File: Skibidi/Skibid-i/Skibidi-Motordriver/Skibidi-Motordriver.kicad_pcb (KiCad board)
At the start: 2 copper layers, 65.5 x 94 mm, 13 parts, among them J1 XT90, J2 XT90, J5 XT90, J7 Screw_Terminal_01x02, J8 Screw_Terminal_01x02, Q1 IGBT, Q2 IGBT, Q3 IGBT, Q4 IGBT, Q5 IGBT, Q6 IGBT, Q7 IGBT, Q8 IGBT

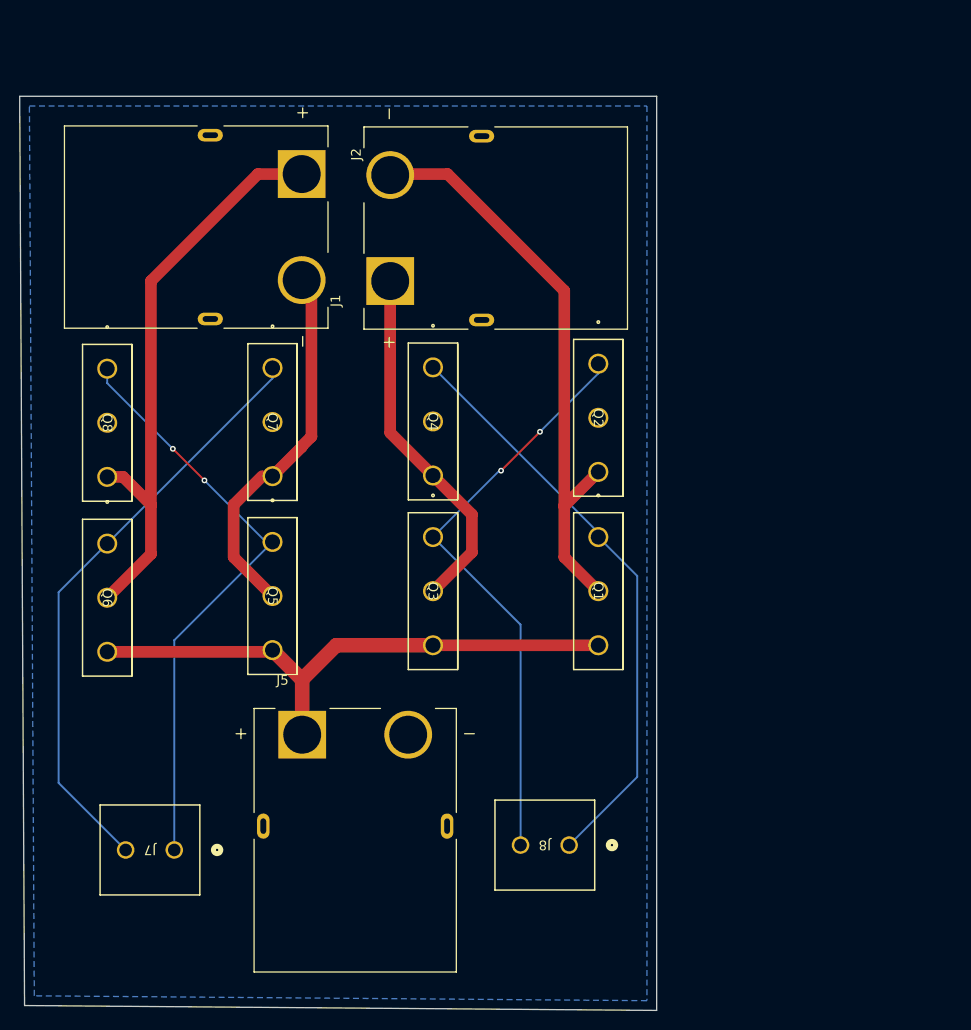
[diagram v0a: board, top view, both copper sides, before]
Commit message: finish motor driver
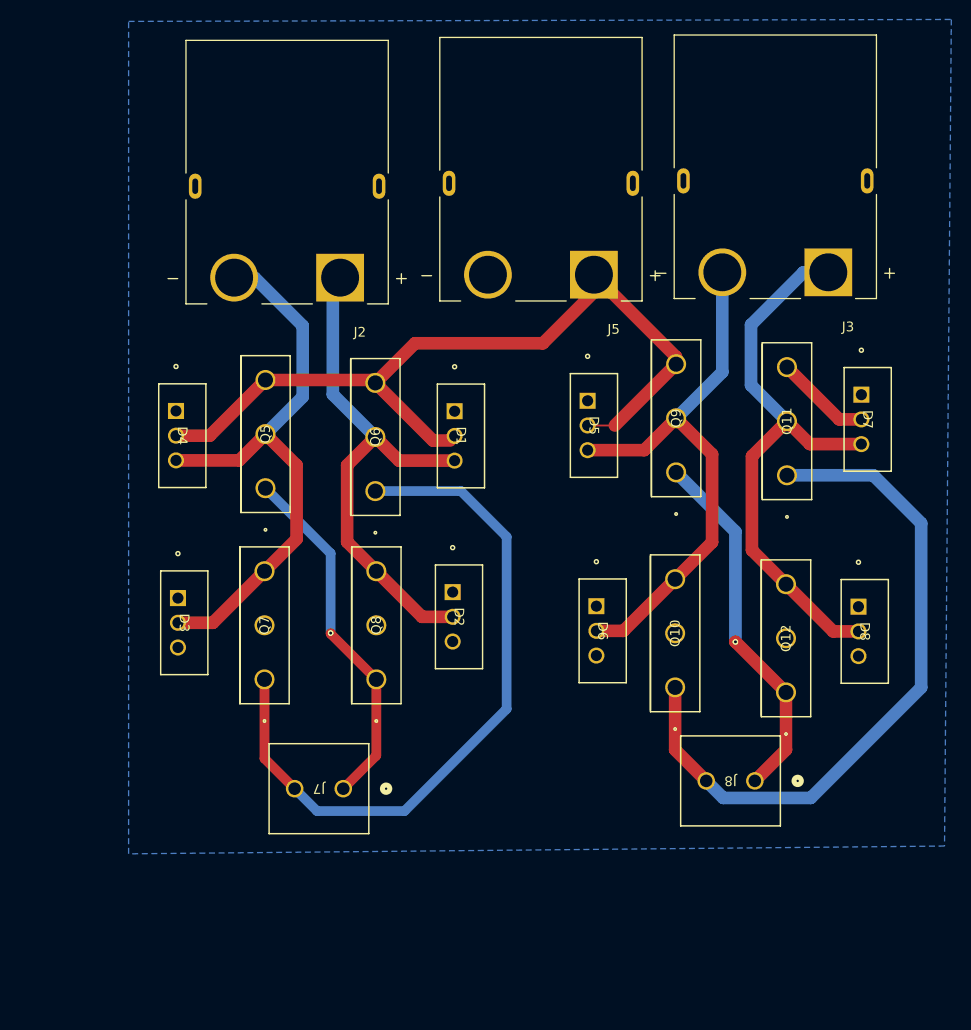
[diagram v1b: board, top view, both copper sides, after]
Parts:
- removed J1: XT90, Skibidi-feet:xt90Female
- removed Q1, Q2, Q3, Q4: IGBT, Skibidi-feet:IGBT
- added D1: D_Schottky_AKA, Skibidi-feet:SchottkyDiode, F.Cu at (162.7, 74.4)
- added D2: D_Schottky_AKA, Skibidi-feet:SchottkyDiode, F.Cu at (162.5, 93.0)
- added D3: D_Schottky_AKA, Skibidi-feet:SchottkyDiode, F.Cu at (134.3, 93.6)
- added D4: D_Schottky_AKA, Skibidi-feet:SchottkyDiode, F.Cu at (134.1, 74.4)
- added D5: D_Schottky_AKA, Skibidi-feet:SchottkyDiode, F.Cu at (176.4, 73.3)
- added D6: D_Schottky_AKA, Skibidi-feet:SchottkyDiode, F.Cu at (177.3, 94.4)
- added D7: D_Schottky_AKA, Skibidi-feet:SchottkyDiode, F.Cu at (204.6, 72.7)
- added D8: D_Schottky_AKA, Skibidi-feet:SchottkyDiode, F.Cu at (204.2, 94.5)
- added J3: XT90, Skibidi-feet:xt90Female, F.Cu at (195.7, 50.7)
- added Q10: IGBT, Skibidi-feet:IGBT, F.Cu at (185.4, 102.8)
- added Q11: IGBT, Skibidi-feet:IGBT, F.Cu at (196.9, 81.0)
- added Q12: IGBT, Skibidi-feet:IGBT, F.Cu at (196.8, 103.3)
- added Q9: IGBT, Skibidi-feet:IGBT, F.Cu at (185.5, 80.7)
- moved J5 68.8 mm to (171.6, 51.0), turned to 180 degrees
- moved Q8 42.3 mm to (154.7, 102.0), turned to 90 degrees
- moved Q7 32.0 mm to (143.2, 102.0), turned to 90 degrees
- moved Q6 28.1 mm to (154.6, 82.6), turned to 90 degrees
- moved J8 20.2 mm to (193.6, 112.4)
- moved J7 18.5 mm to (151.3, 113.2)
- moved J2 8.95 mm to (145.5, 51.2), turned to 180 degrees
- moved Q5 5.57 mm to (143.3, 82.3), turned to 90 degrees
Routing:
- net Net-(J1-NEG): track 60.2 -> 0.00 mm
- net Net-(D8-K): track 0.00 -> 59.4 mm
- net Net-(D6-K): track 0.00 -> 57.4 mm
- net Net-(J1-POS): track 37.0 -> 0.00 mm
- net +48V: track 59.7 -> 96.2 mm
- net BDC11: track 61.1 -> 37.0 mm, vias 2 -> 1
- net BDC1: track 60.7 -> 37.7 mm, vias 0 -> 1
- net Net-(D3-K): track 38.5 -> 60.0 mm
- net BDC22: track 61.5 -> 72.8 mm
- net BDC2: track 60.4 -> 71.2 mm, vias 2 -> 0
- net Net-(D2-K): track 60.2 -> 53.7 mm
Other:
- board outline removed
